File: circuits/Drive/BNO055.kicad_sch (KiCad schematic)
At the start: 6 parts, among them Q1 BSS138, U13 BNO055

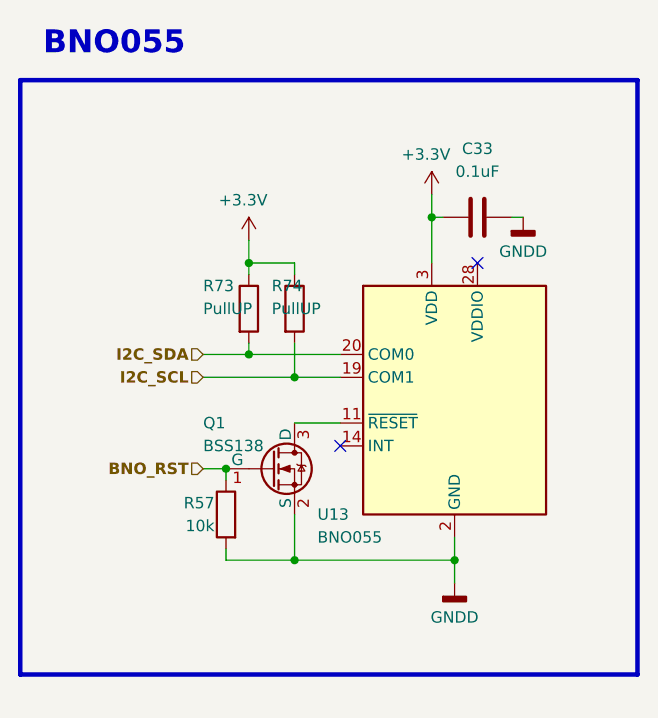
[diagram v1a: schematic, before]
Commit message: 無線&UI完成？
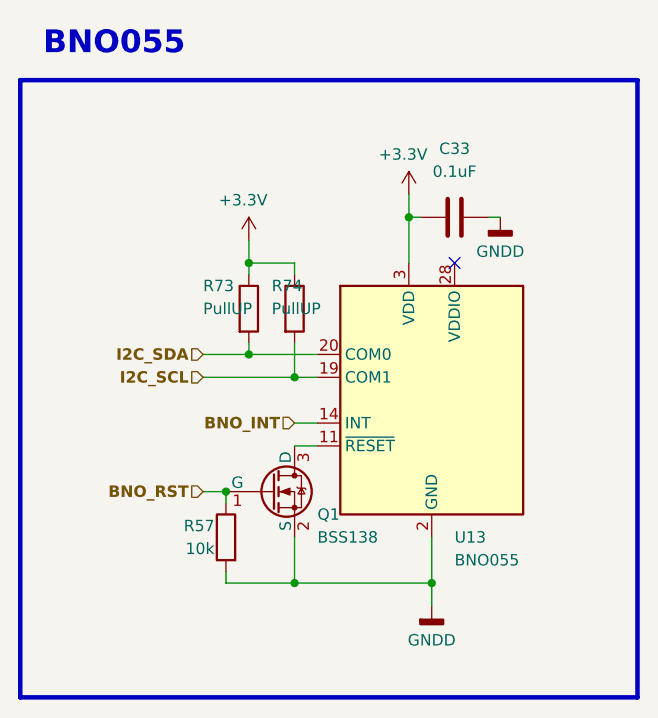
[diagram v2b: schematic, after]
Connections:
- net BNO_INT: now reaches U13.14 (INT)
- no-connect marks 2 -> 1
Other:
- moved on the sheet: C33, Q1, R57, U13

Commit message: ラズパイ基板とか
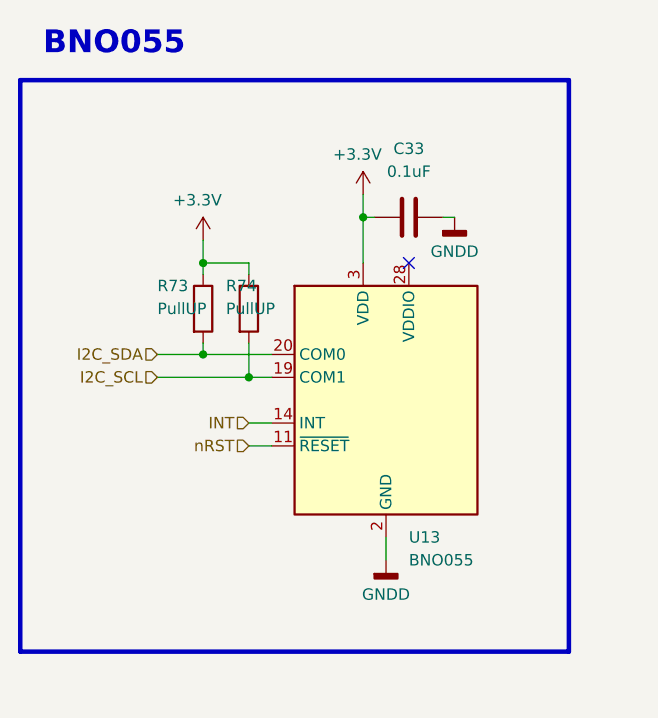
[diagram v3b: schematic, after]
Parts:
- removed Q1: BSS138, Package_TO_SOT_SMD:SOT-23, symbol Device:Q_NMOS_GSD
- removed R57: 10k, Resistor_SMD:R_0402_1005Metric, symbol Device:R
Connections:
- net nRST: now reaches U13.11 (~{RESET})
- net BNO_INT renamed INT
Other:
- moved on the sheet: C33, R73, R74, U13

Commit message: シンボル・フットプリントMyLib->TomoshibiLib置き換え
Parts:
- U13: footprint MyLibrary:Sensor_Motion_Aktk_BNO055 -> TomoshibiLibrary:Sensor_Motion_Aktk_BNO055
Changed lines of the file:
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@@
       (effects (font (size 1.27 1.27)) (justify left))
     )
-    (property "Footprint" "MyLibrary:Sensor_Motion_Aktk_BNO055" (at 158.75 100.33 0)
+    (property "Footprint" "TomoshibiLibrary:Sensor_Motion_Aktk_BNO055" (at 158.75 100.33 0)
       (effects (font (size 1.27 1.27)) (justify left) hide)
     )
